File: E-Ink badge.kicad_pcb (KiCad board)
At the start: 2 copper layers, 80.8 x 63.8 mm, 40 parts, among them J1 USB_C_Receptacle_USB2.0_14P, J2 E-INK-FPC, Q1 BSS138, SW1 BOOTSEL, SW2 RUN, SW3 W, SW4 A, SW5 S, SW6 D, U1 RP2040, U2 AP2112K-3.3, U3 W25Q16JVSS, Y1 Crystal

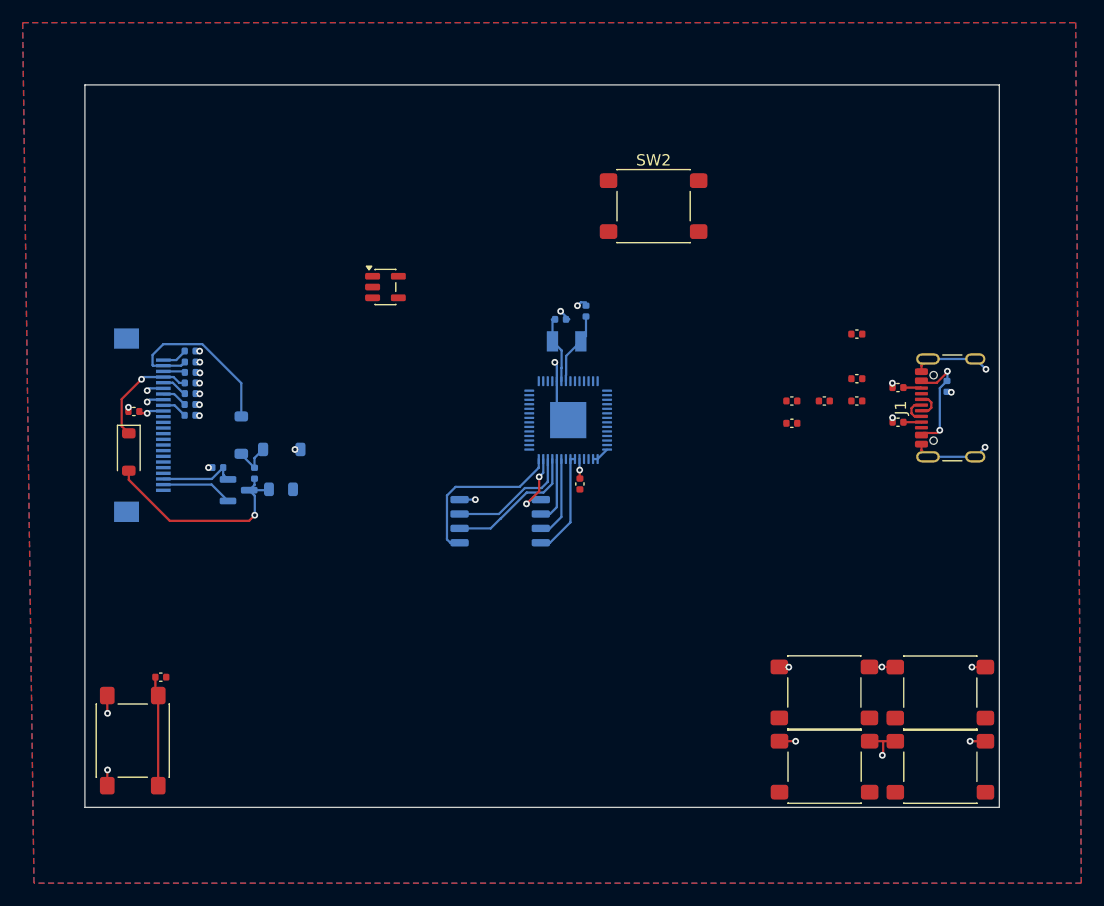
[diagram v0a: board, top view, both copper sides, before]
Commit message: Finally finished routing the whole board!
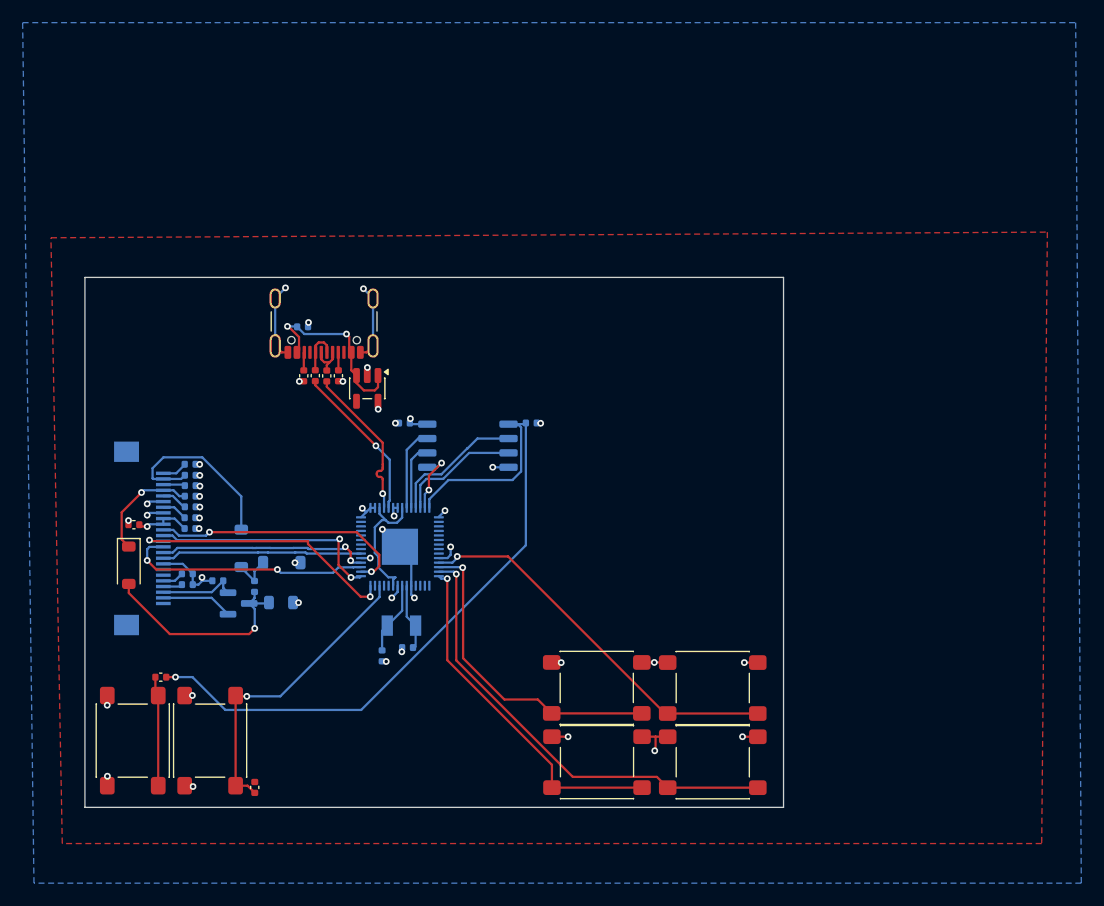
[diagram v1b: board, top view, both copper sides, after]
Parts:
- C15, C6, C7, R4: moved to B.Cu
- moved R6 64.3 mm to (133.5, 131.5), turned to 90 degrees
- moved SW2 61.3 mm to (129.6, 127.4), turned to 90 degrees
- moved C1 57.2 mm to (137.7, 90.9), turned to 180 degrees
- moved J1 57.1 mm to (139.6, 89.4), turned to 180 degrees
- moved C6 55.5 mm to (127.5, 112.7), turned to 180 degrees
- moved C7 55.3 mm to (127.5, 113.6), turned to 180 degrees
- moved R3 52.5 mm to (137.8, 95.2), turned to -90 degrees
- moved R2 49.6 mm to (140.9, 95.2), turned to -90 degrees
- moved R7 46.9 mm to (139.9, 95.2), turned to -90 degrees
- moved C15 37.1 mm to (146.7, 99.4), turned to 180 degrees
- moved C14 35.4 mm to (144.7, 119.9), turned to -90 degrees
- moved C13 32.0 mm to (147.0, 119.2), turned to 180 degrees
- moved R4 29.8 mm to (157.9, 99.4), turned to 180 degrees
- moved Y1 29.0 mm to (146.5, 117.2), turned to 0 degrees
- moved R8 25.3 mm to (138.8, 95.2), turned to 90 degrees
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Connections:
- U1 pad 11: unconnected-(U1-GPIO8-Pad11) -> GPIO_W
- U1 pad 12: unconnected-(U1-GPIO9-Pad12) -> GPIO_A
- U1 pad 13: unconnected-(U1-GPIO10-Pad13) -> GPIO_D
- U1 pad 14: unconnected-(U1-GPIO11-Pad14) -> GPIO_S
- U1 pad 2: GPIO_W -> unconnected-(U1-GPIO0-Pad2)
- U1 pad 3: GPIO_A -> unconnected-(U1-GPIO1-Pad3)
- U1 pad 4: GPIO_S -> unconnected-(U1-GPIO2-Pad4)
- U1 pad 5: GPIO_D -> unconnected-(U1-GPIO3-Pad5)
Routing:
- net BOOTSEL: track 15.0 -> 66.4 mm, vias 0 -> 1
- net GPIO_D: track 0.00 -> 40.5 mm, vias 0 -> 1
- net GPIO_W: track 0.00 -> 34.4 mm, vias 0 -> 1
- net GPIO_S: track 0.00 -> 31.1 mm, vias 0 -> 1
- net GPIO_A: track 0.00 -> 27.9 mm, vias 0 -> 1
- net RUN: track 0.00 -> 27.3 mm, vias 0 -> 1
- net CS: track 0.00 -> 24.0 mm, vias 0 -> 2
- net MOSI: track 0.00 -> 23.1 mm, vias 0 -> 2
- net DC: track 0.00 -> 22.0 mm, vias 0 -> 2
- net CLK: track 0.00 -> 20.6 mm, vias 0 -> 2
- net RST: track 0.00 -> 18.8 mm, vias 0 -> 2
- net BUSY: track 0.00 -> 17.7 mm
- net Net-(U1-USB_DM): track 0.00 -> 13.9 mm, vias 0 -> 1
- net Net-(U1-USB_DP): track 1.74 -> 14.0 mm
- net Net-(U1-VREG_VOUT): track 0.00 -> 11.5 mm
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- added copper zone on F.Cu, net +3.3V
- removed copper zone on F.Cu, net GND
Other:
- board size 80.8 x 63.8 mm -> 61.7 x 46.8 mm
- board text added: "W A S D"
